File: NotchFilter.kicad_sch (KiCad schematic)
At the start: 11 parts, among them U4 LM2904DR

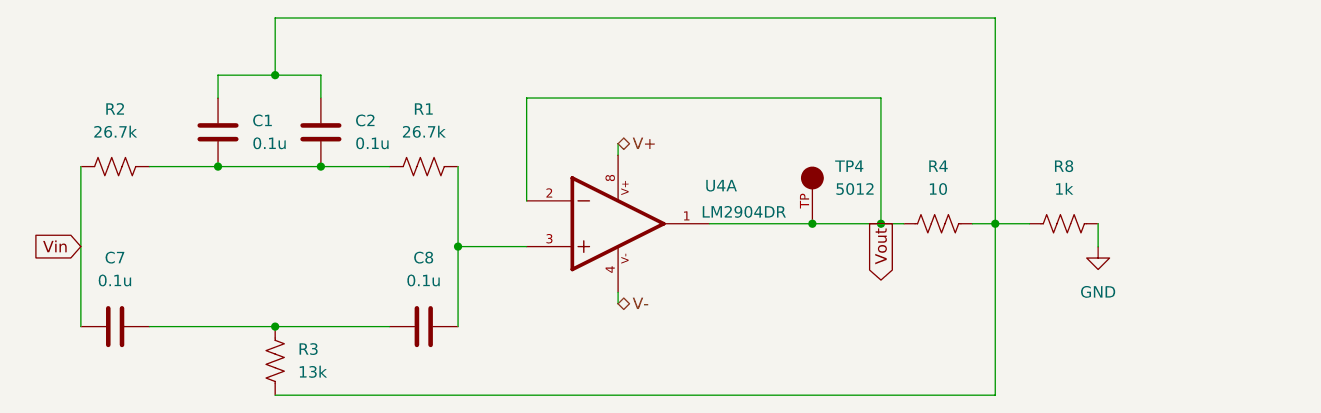
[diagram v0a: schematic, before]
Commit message: merge fix 2
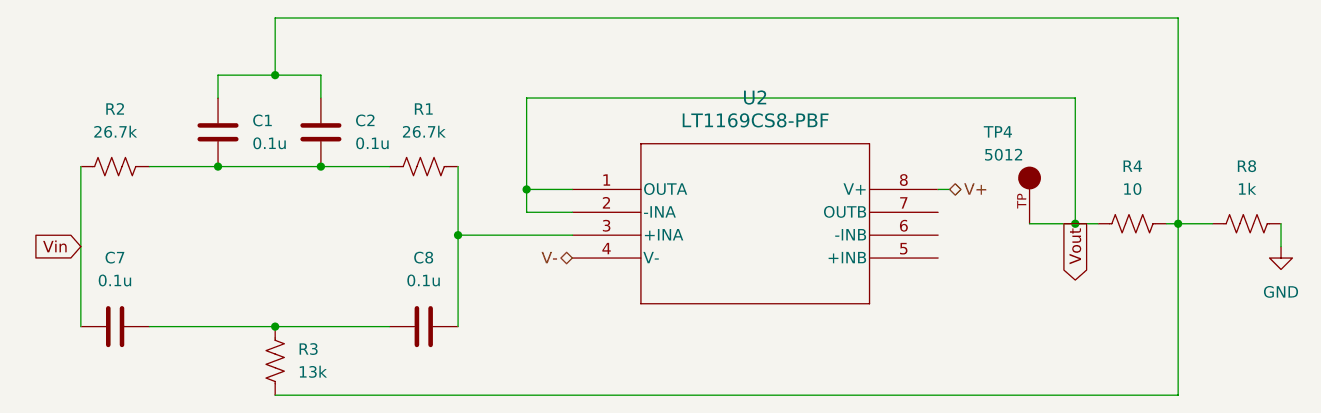
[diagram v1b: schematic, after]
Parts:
- removed U4: LM2904DR, LM2904DR:SOIC127P599X175-8N, symbol LM2904DR:LM2904DR
- added U2: LT1169CS8-PBF, SO-8_S_LIT, symbol symbols:LT1169CS8-PBF
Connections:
- net V+: now also U2.8 (V+)
- net V-: now also U2.4 (V-)
- net Vout: now also U2.1 (OUTA), U2.2 (-INA)
- net at C8.2, R1.2: now also U2.3 (+INA)
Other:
- moved on the sheet: R4, R8, TP4
